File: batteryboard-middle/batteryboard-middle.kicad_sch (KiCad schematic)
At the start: 8 parts, among them J1 Conn_02x05_Odd_Even, J2 Conn_01x02, J3 Conn_01x02, J4 Conn_02x05_Odd_Even

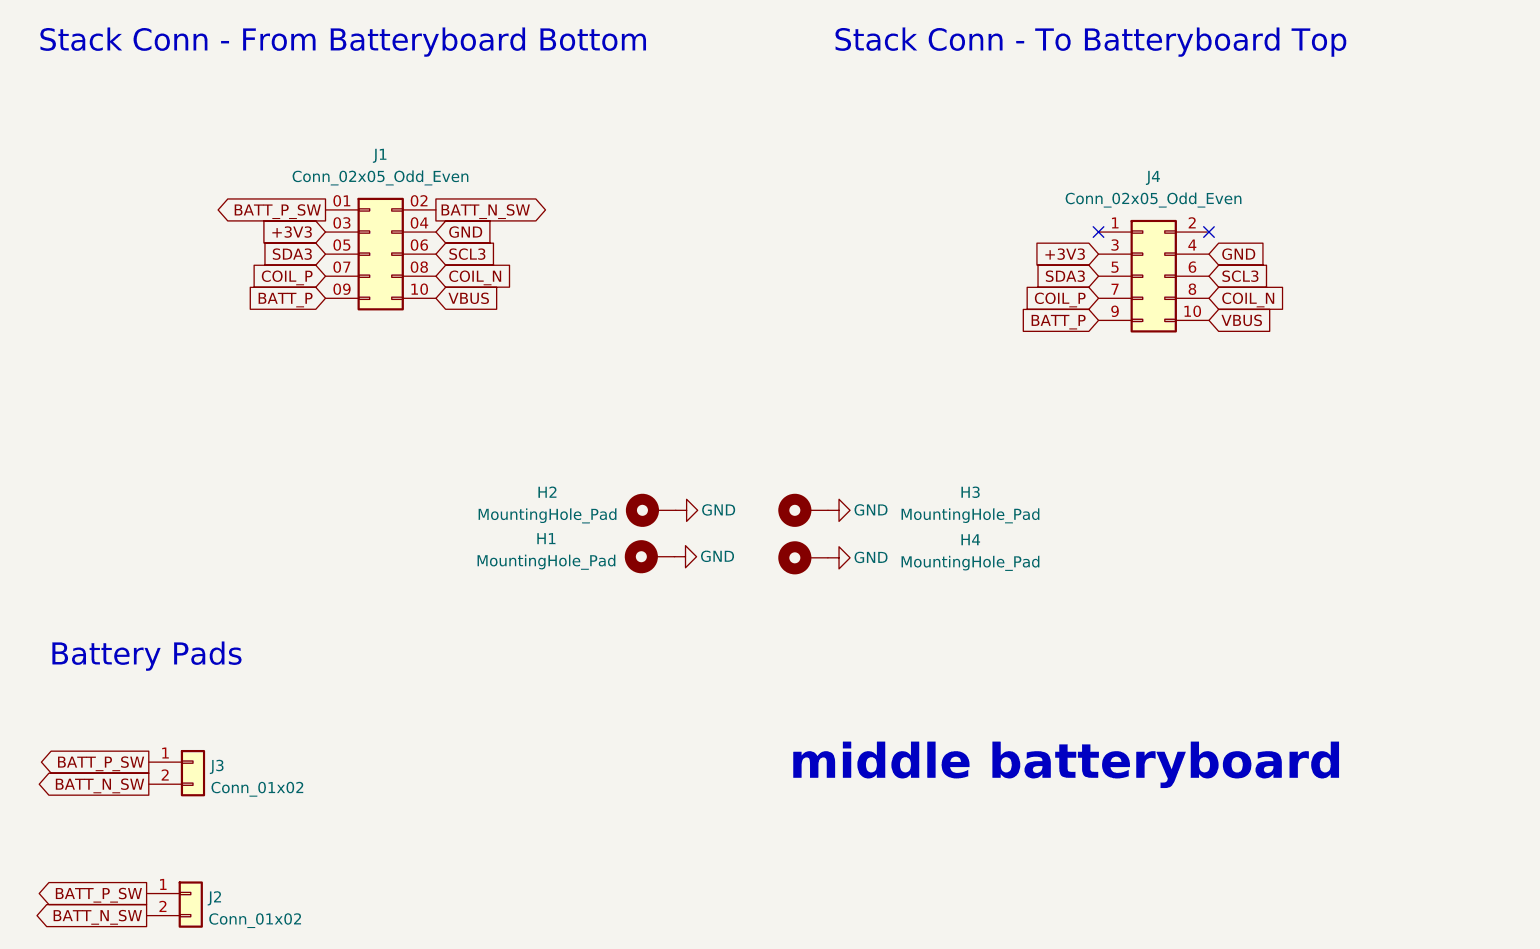
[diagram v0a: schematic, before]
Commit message: Recheck boards and re-export models
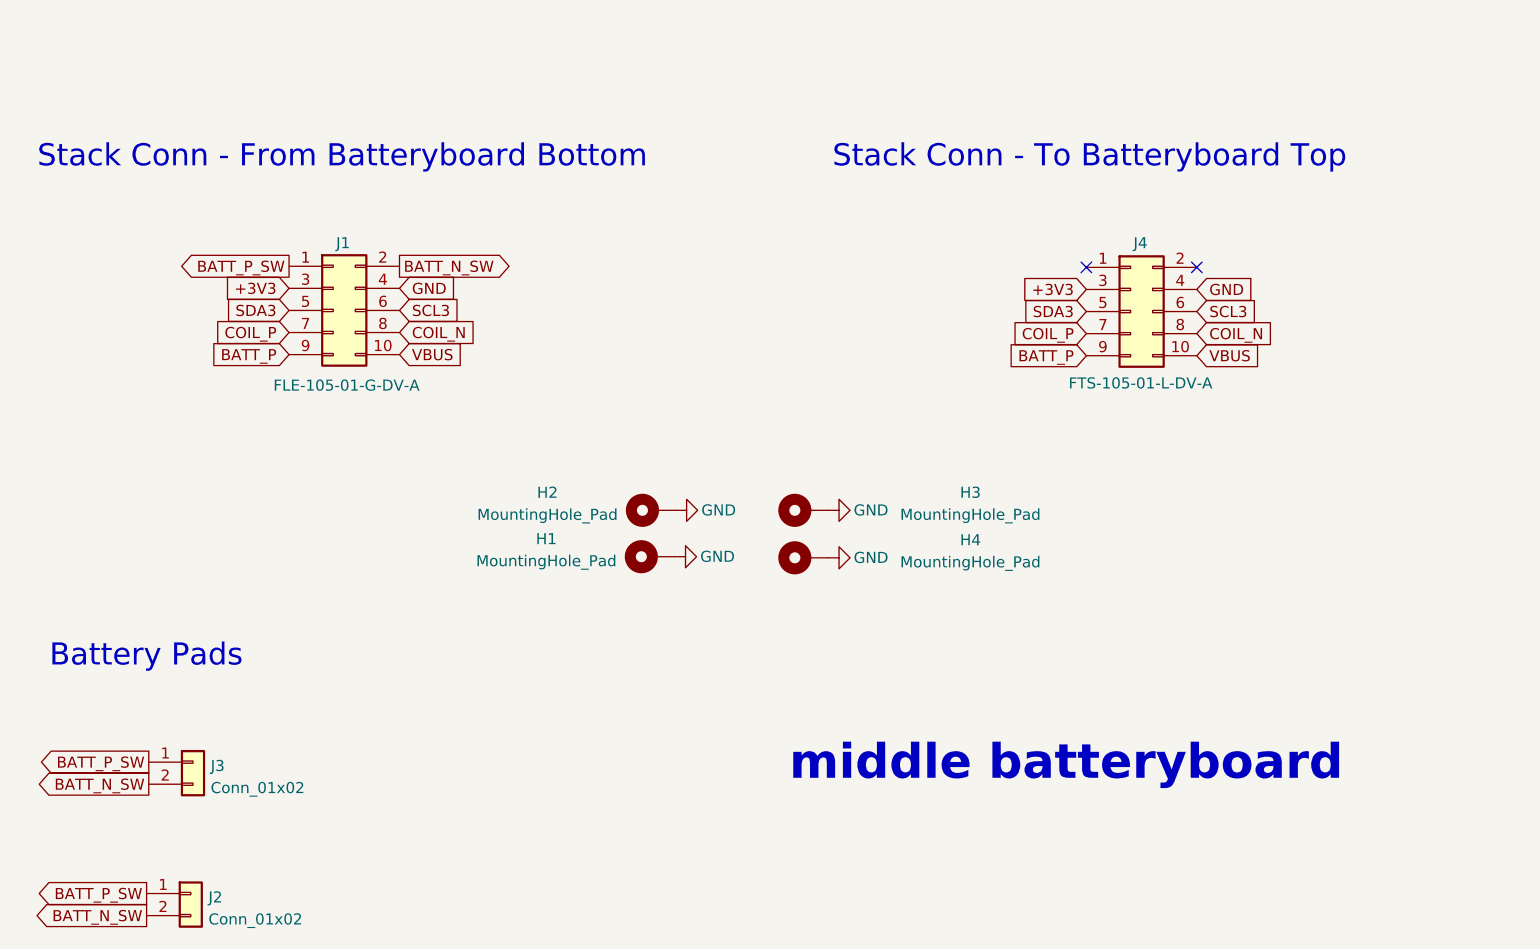
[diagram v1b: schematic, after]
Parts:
- J1: value Conn_02x05_Odd_Even -> FLE-105-01-G-DV-A
- J4: value Conn_02x05_Odd_Even -> FTS-105-01-L-DV-A
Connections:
- net +3V3: now also J1.3 (Pin_3); no longer J1.03 (Pin_3)
- net BATT_N_SW: now also J1.2 (Pin_2); no longer J1.02 (Pin_2)
- net BATT_P: now also J1.9 (Pin_9); no longer J1.09 (Pin_9)
- net BATT_P_SW: now also J1.1 (Pin_1); no longer J1.01 (Pin_1)
- net COIL_N: now also J1.8 (Pin_8); no longer J1.08 (Pin_8)
- net COIL_P: now also J1.7 (Pin_7); no longer J1.07 (Pin_7)
- net GND: now also J1.4 (Pin_4); no longer J1.04 (Pin_4)
- net SCL3: now also J1.6 (Pin_6); no longer J1.06 (Pin_6)
- net SDA3: now also J1.5 (Pin_5); no longer J1.05 (Pin_5)
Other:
- moved on the sheet: J1, J4
